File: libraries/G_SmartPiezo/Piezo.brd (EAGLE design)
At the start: 25.5 x 32 mm, 13 parts, among them U1 ATMEGA328

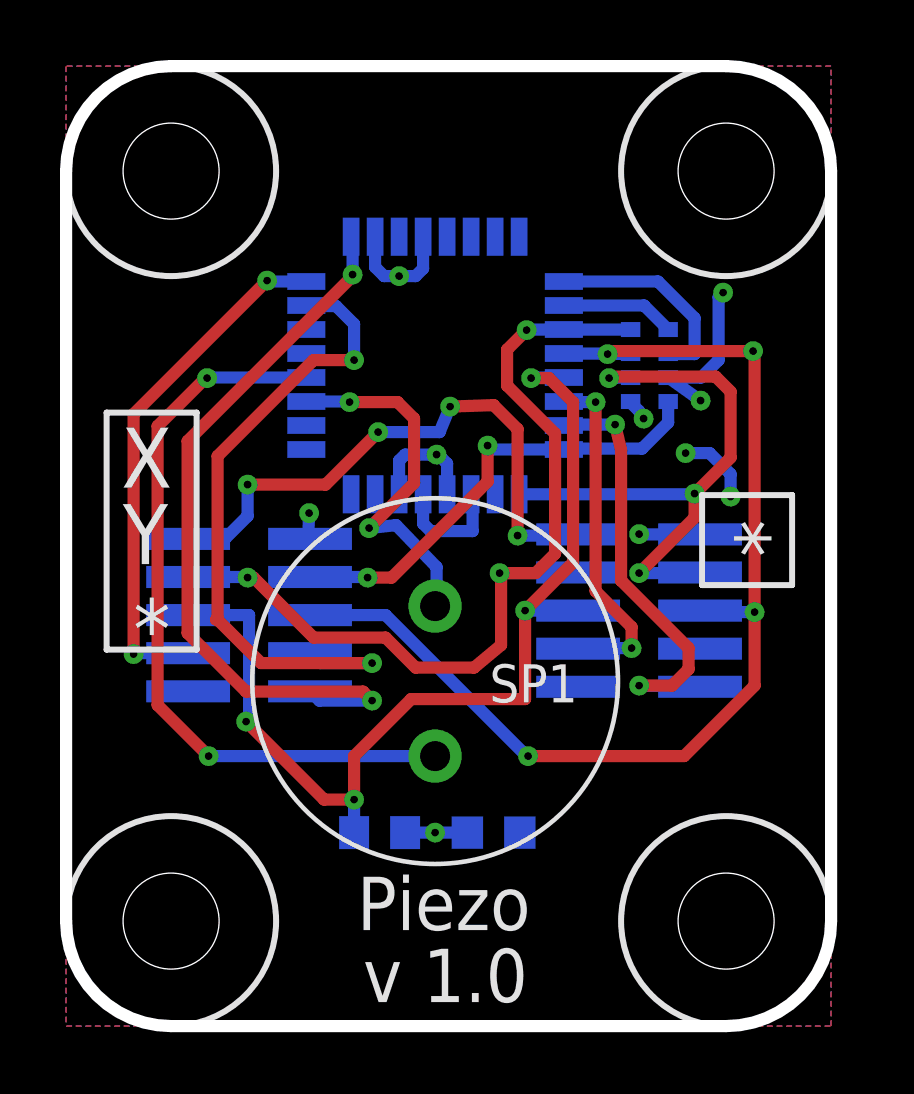
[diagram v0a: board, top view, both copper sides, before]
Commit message: The latest version of the module's eagle files
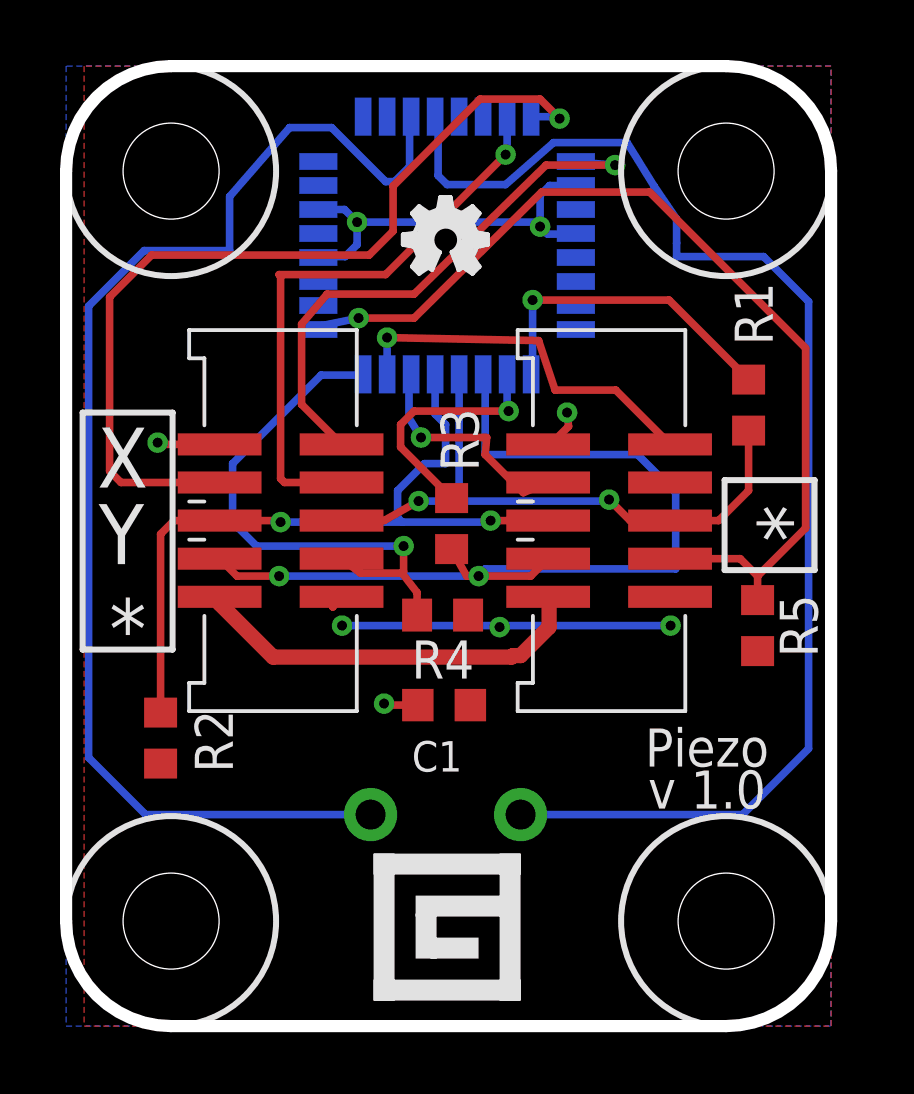
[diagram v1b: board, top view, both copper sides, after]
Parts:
- added R3, R4, R5: 10K, rcl:R0603
- added U$7: (no value), Gadgeteer:GADGETEER_LOGO_SMALL
- added U$8: (no value), Architect:OSHW_LOGO
- R1: device SparkFun:0603-ARV -> rcl:R0603
- moved R2 7.95 mm to (3.15, 9.60), flipped to the top, turned to 270 degrees
- moved C1 4.56 mm to (12.6, 10.7), flipped to the top
- moved SP1 4.46 mm to (12.7, 7.05), flipped to the bottom, turned to 0 degrees
- moved U1 4.02 mm to (12.7, 26.0), turned to 180 degrees
- moved R1 3.56 mm to (22.8, 20.7), flipped to the top
- moved XY 3.32 mm to (7.15, 16.9), flipped to the top, turned to 180 degrees
- moved * 3.16 mm to (18.1, 16.9), flipped to the top, turned to 180 degrees
- moved U$6 0.90 mm to (24.9, 15.2)
- moved U$5 0.80 mm to (0.05, 12.4)
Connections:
- net DN: now also R5.1; no longer R1.6
- net N$1: now also R1.1; no longer R1.2
- net N$2: now also R3.1; no longer R1.1
- net SCL: now also R1.2; no longer R1.7
- net SDA: now also R3.2; no longer R1.8
- net UP: now also R4.1; no longer R1.4
- net VCC: now also R4.2, R5.2; no longer R1.3, R1.5
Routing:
- net SP1: track 12.3 -> 42.2 mm, vias 2 -> 0
- net SP2: track 25.0 -> 43.7 mm, vias 2 -> 0
- net SCL: track 38.7 -> 20.7 mm, vias 4 -> 2
- net DN: track 20.3 -> 32.4 mm, vias 3 -> 1
- net MISO: track 17.4 -> 29.5 mm, vias 2 -> 1
- net RST: track 34.6 -> 25.3 mm, vias 4 -> 2
- net SCK: track 24.8 -> 18.5 mm, vias 2 -> 1
- net +5V: track 19.5 -> 13.4 mm, vias 4 -> 0
- net N$2: track 3.81 -> 8.19 mm, vias 0 -> 1
- net RX: track 11.6 -> 7.69 mm, vias 2 -> 1
- net VCC: track 21.6 -> 25.5 mm, vias 10 -> 5
- net N$1: track 6.95 -> 10.8 mm, vias 0 -> 1
- net MOSI: track 22.4 -> 19.4 mm, vias 2 -> 1
- net UP: track 15.6 -> 18.2 mm, vias 2 -> 1
- net TX: track 14.8 -> 12.6 mm, vias 2 -> 1
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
